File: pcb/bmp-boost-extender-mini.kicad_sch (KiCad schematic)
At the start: 2 parts

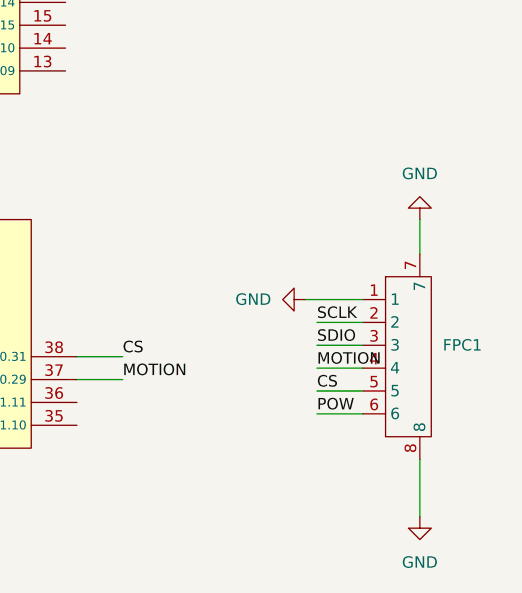
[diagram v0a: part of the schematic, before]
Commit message: minor fix
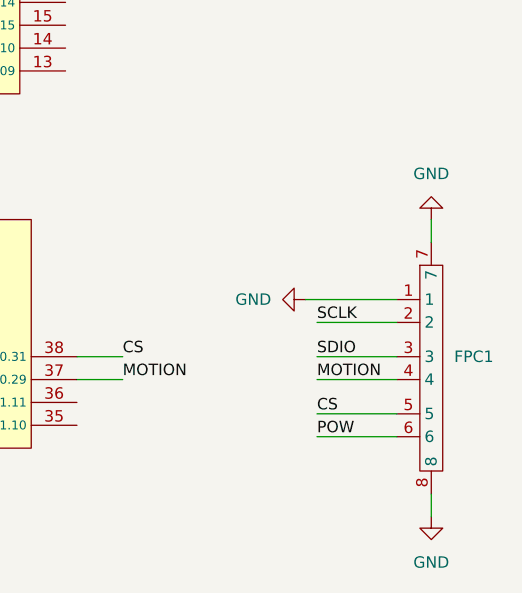
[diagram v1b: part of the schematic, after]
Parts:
- removed FPC1: ~, Library:FPC-SMD_6P-P0.50_GT-F0501SR10-06S1101, symbol New_Library:GT-F0501SR10-06S1101
- added FPC1: ~, Library:FPC-SMD_6P-P0.50_GT-F0501SR10-06S1101, symbol conn_6p:GT-F0501SR10-06S1101
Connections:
- net CS: now also FPC1.5
- net GND: now also FPC1.1, FPC1.7, FPC1.8
- net MOTION: now also FPC1.4
- net POW: now also FPC1.6
- net SCLK: now also FPC1.2
- net SDIO: now also FPC1.3
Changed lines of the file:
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@@
 	(wire
 		(pts
-			(xy 144.78 105.41) (xy 149.86 105.41)
-		)
-		(stroke
-			(width 0)
-			(type default)
-		)
-	)
-	(wire
-		(pts
-			(xy 156.21 83.82) (xy 156.21 87.63)
+			(xy 144.78 107.95) (xy 153.67 107.95)
+		)
+		(stroke
+			(width 0)
+			(type default)
+		)
+	)
+	(wire
+		(pts
+			(xy 157.48 83.82) (xy 157.48 86.36)
 		)
 		(stroke
@@
 	(wire
 		(pts
-			(xy 144.78 102.87) (xy 149.86 102.87)
+			(xy 144.78 105.41) (xy 153.67 105.41)
 		)
 		(stroke
@@
 	(wire
 		(pts
-			(xy 143.51 92.71) (xy 149.86 92.71)
-		)
-		(stroke
-			(width 0)
-			(type default)
-		)
-	)
-	(wire
-		(pts
-			(xy 144.78 95.25) (xy 149.86 95.25)
-		)
-		(stroke
-			(width 0)
-			(type default)
-		)
-	)
-	(wire
-		(pts
-			(xy 144.78 97.79) (xy 149.86 97.79)
+			(xy 143.51 92.71) (xy 153.67 92.71)
+		)
+		(stroke
+			(width 0)
+			(type default)
+		)
+	)
+	(wire
+		(pts
+			(xy 144.78 95.25) (xy 153.67 95.25)
+		)
+		(stroke
+			(width 0)
+			(type default)
+		)
+	)
+	(wire
+		(pts
+			(xy 144.78 99.06) (xy 153.67 99.06)
 		)
 		(stroke
@@
 	(wire
 		(pts
-			(xy 156.21 110.49) (xy 156.21 116.84)
-		)
-		(stroke
-			(width 0)
-			(type default)
-		)
-	)
-	(wire
-		(pts
 			(xy 85.09 93.98) (xy 90.17 93.98)
 		)
@@
 	(wire
 		(pts
-			(xy 144.78 100.33) (xy 149.86 100.33)
+			(xy 157.48 114.3) (xy 157.48 116.84)
+		)
+		(stroke
+			(width 0)
+			(type default)
+		)
+	)
+	(wire
+		(pts
+			(xy 144.78 101.6) (xy 153.67 101.6)
 		)
 		(stroke
@@
 	)
 	(label "CS"
-		(at 144.78 102.87 0)
+		(at 144.78 105.41 0)
 		(effects
 			(font
@@
 	)
 	(label "MOTION"
-		(at 144.78 100.33 0)
+		(at 144.78 101.6 0)
 		(effects
 			(font
@@
 	)
 	(label "POW"
-		(at 144.78 105.41 0)
+		(at 144.78 107.95 0)
 		(effects
 			(font
@@
 	)
 	(label "SDIO"
-		(at 144.78 97.79 0)
+		(at 144.78 99.06 0)
 		(effects
 			(font
@@
 			)
 			(justify left bottom)
-		)
-	)
-	(symbol
-		(lib_id "New_Library:GT-F0501SR10-06S1101")
-		(at 153.67 99.06 0)
-		(unit 1)
-		(exclude_from_sim no)
-		(in_bom yes)
-		(on_board yes)
-		(dnp no)
-		(fields_autoplaced yes)
-		(property "Reference" "FPC1"
-			(at 158.75 97.7899 0)
-			(effects
-				(font
-					(size 1.27 1.27)
-				)
-				(justify left)
-			)
-		)
-		(property "Value" "~"
-			(at 158.75 100.3299 0)
-			(effects
-				(font
-					(size 1.27 1.27)
-				)
-				(justify left)
-			)
-		)
-		(property "Footprint" "Library:FPC-SMD_6P-P0.50_GT-F0501SR10-06S1101"
-			(at 151.892 117.094 0)
-			(effects
-				(font
-					(size 1.27 1.27)
-				)
-				(hide yes)
-			)
-		)
-		(property "Datasheet" "https://item.szlcsc.com/datasheet/GT-F0501SR10-06S1101/23912640.html"
-			(at 152.4 127.508 0)
-			(effects
-				(font
-					(size 1.27 1.27)
-				)
-				(hide yes)
-			)
-		)
-		(property "Description" "Locking Feature:Hinged Lid Contact Type:Bottom Contact Number of Contacts:6P Pitch:0.5mm Mounting Type:Surface Mount, Right Angle FFC, FCB Thickness:0.3mm FFC, FCB Thickness:0.3mm Height Above Board:1mm Contact Material:Phosphor Bronze Contact Plating:Gol"
-			(at 151.638 121.92 0)
-			(effects
-				(font
-					(size 1.27 1.27)
-				)
-				(hide yes)
-			)
-		)
-		(property "Manufacturer Part" "GT-F0501SR10-06S1101"
-			(at 151.384 124.206 0)
-			(effects
-				(font
-					(size 1.27 1.27)
-				)
-				(hide yes)
-			)
-		)
-		(property "Manufacturer" "G-Switch(品赞)"
-			(at 156.21 77.978 0)
-			(effects
-				(font
-					(size 1.27 1.27)
-				)
-				(hide yes)
-			)
-		)
-		(property "Supplier Part" "C22380676"
-			(at 160.274 80.772 0)
-			(effects
-				(font
-					(size 1.27 1.27)
-				)
-				(hide yes)
-			)
-		)
-		(property "Supplier" "LCSC"
-			(at 173.228 85.09 0)
-			(effects
-				(font
-					(size 1.27 1.27)
-				)
-				(hide yes)
-			)
-		)
-		(property "LCSC Part Name" "翻盖式 下接 P数:6P 间距:0.5mm"
-			(at 151.892 119.888 0)
-			(effects
-				(font
-					(size 1.27 1.27)
-				)
-				(hide yes)
-			)
-		)
-		(pin "1"
-		)
-		(pin "3"
-		)
-		(pin "4"
-		)
-		(pin "2"
-		)
-		(pin "5"
-		)
-		(pin "6"
-		)
-		(pin "7"
-		)
-		(pin "8"
-		)
-		(instances
-			(project ""
-				(path "/815c08ea-bf5d-4627-a659-f0b77cf7dff8"
-					(reference "FPC1")
-					(unit 1)
-				)
-			)
 		)
 	)
@@
 	(symbol
 		(lib_id "Library:GND")
-		(at 156.21 116.84 0)
+		(at 157.48 116.84 0)
 		(unit 1)
 		(exclude_from_sim no)
@@
 		(fields_autoplaced yes)
 		(property "Reference" "#PWR03"
-			(at 156.21 123.19 0)
+			(at 157.48 123.19 0)
 			(effects
 				(font
@@
 		)
 		(property "Value" "GND"
-			(at 156.21 121.92 0)
+			(at 157.48 121.92 0)
 			(effects
 				(font
@@
 		)
 		(property "Footprint" ""
-			(at 156.21 116.84 0)
+			(at 157.48 116.84 0)
 			(effects
 				(font
@@
 		)
 		(property "Datasheet" ""
-			(at 156.21 116.84 0)
+			(at 157.48 116.84 0)
 			(effects
 				(font
@@
 		)
 		(property "Description" "Power symbol creates a global label with name \"GND\" , ground"
-			(at 156.21 116.84 0)
+			(at 157.48 116.84 0)
 			(effects
 				(font
@@
 	)
 	(symbol
+		(lib_id "conn_6p:GT-F0501SR10-06S1101")
+		(at 157.48 100.33 0)
+		(unit 1)
+		(exclude_from_sim no)
+		(in_bom yes)
+		(on_board yes)
+		(dnp no)
+		(fields_autoplaced yes)
+		(property "Reference" "FPC1"
+			(at 160.02 99.0599 0)
+			(effects
+				(font
+					(size 1.27 1.27)
+				)
+				(justify left)
+			)
+		)
+		(property "Value" "~"
+			(at 160.02 101.5999 0)
+			(effects
+				(font
+					(size 1.27 1.27)
+				)
+				(justify left)
+			)
+		)
+		(property "Footprint" "Library:FPC-SMD_6P-P0.50_GT-F0501SR10-06S1101"
+			(at 155.702 118.364 0)
+			(effects
+				(font
+					(size 1.27 1.27)
+				)
+				(hide yes)
+			)
+		)
+		(property "Datasheet" ""
+			(at 156.21 128.778 0)
+			(effects
+				(font
+					(size 1.27 1.27)
+				)
+				(hide yes)
+			)
+		)
+		(property "Description" ""
+			(at 155.448 123.19 0)
+			(effects
+				(font
+					(size 1.27 1.27)
+				)
+				(hide yes)
+			)
+		)
+		(pin "1"
+		)
+		(pin "2"
+		)
+		(pin "6"
+		)
+		(pin "7"
+		)
+		(pin "8"
+		)
+		(pin "5"
+		)
+		(pin "3"
+		)
+		(pin "4"
+		)
+		(instances
+			(project ""
+				(path "/815c08ea-bf5d-4627-a659-f0b77cf7dff8"
+					(reference "FPC1")
+					(unit 1)
+				)
+			)
+		)
+	)
+	(symbol
 		(lib_id "BMP-Boost:BMP-Boost")
 		(at 102.87 34.29 0)
@@
 	(symbol
 		(lib_id "Library:GND")
-		(at 156.21 83.82 180)
+		(at 157.48 83.82 180)
 		(unit 1)
 		(exclude_from_sim no)
@@
 		(fields_autoplaced yes)
 		(property "Reference" "#PWR02"
-			(at 156.21 77.47 0)
+			(at 157.48 77.47 0)
 			(effects
 				(font
@@
 		)
 		(property "Value" "GND"
-			(at 156.21 78.74 0)
+			(at 157.48 78.74 0)
 			(effects
 				(font
@@
 		)
 		(property "Footprint" ""
-			(at 156.21 83.82 0)
+			(at 157.48 83.82 0)
 			(effects
 				(font
@@
 		)
 		(property "Datasheet" ""
-			(at 156.21 83.82 0)
+			(at 157.48 83.82 0)
 			(effects
 				(font
@@
 		)
 		(property "Description" "Power symbol creates a global label with name \"GND\" , ground"
-			(at 156.21 83.82 0)
-			(effects
-				(font
+			(at 157.48 83.82 0)
+			(effects
+				(font
